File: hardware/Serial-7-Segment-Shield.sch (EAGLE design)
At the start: 32 parts, among them J1 AVR_SPI_PRG_6PTH, U1 ARDUINO_SHIELDLABEL

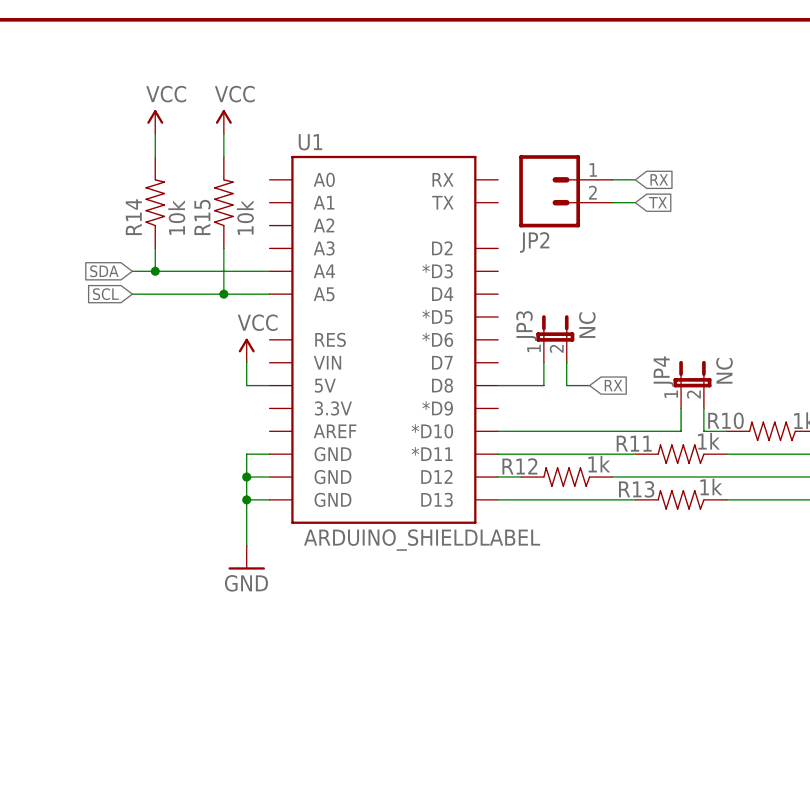
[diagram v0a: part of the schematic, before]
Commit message: commit to QC branch
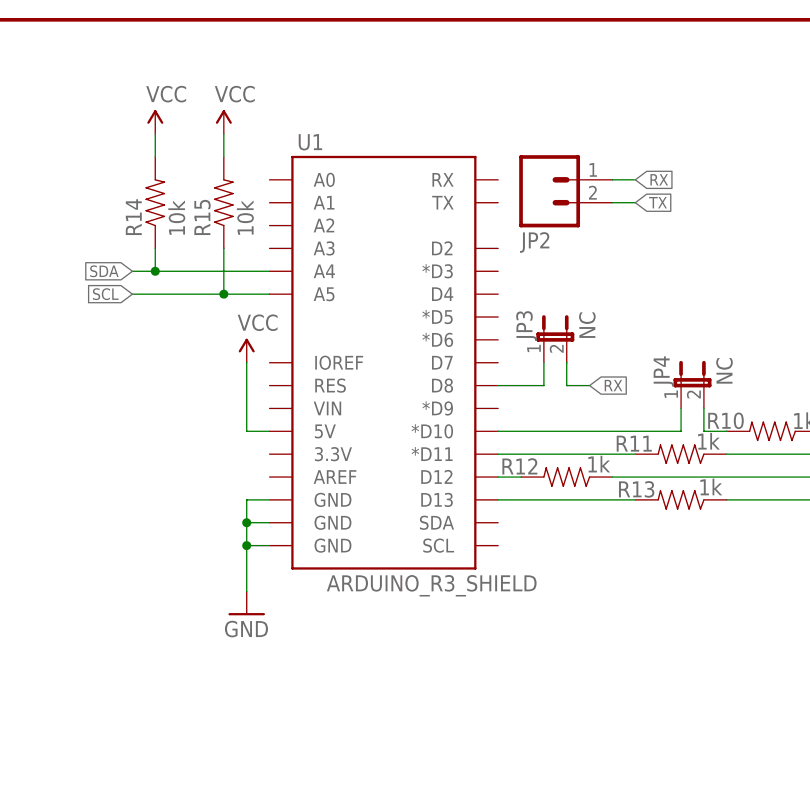
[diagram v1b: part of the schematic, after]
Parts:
- U1: value ARDUINO_SHIELDLABEL -> ARDUINO_R3_SHIELD; device SparkFun-Boards:ARDUINO_SHIELDLABEL -> SparkFun-Boards:ARDUINO_R3_SHIELD
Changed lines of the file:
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@@
 <?xml version="1.0" encoding="utf-8"?>
 <!DOCTYPE eagle SYSTEM "eagle.dtd">
-<eagle version="6.5.0">
+<eagle version="6.4">
 <drawing>
 <settings>
@@
 <part name="JP9" library="SparkFun" deviceset="FIDUCIAL" device="UFIDUCIAL"/>
 <part name="JP10" library="SparkFun" deviceset="FIDUCIAL" device="UFIDUCIAL"/>
-<part name="U1" library="SparkFun-Boards" deviceset="ARDUINO_SHIELD" device="LABEL"/>
+<part name="U1" library="SparkFun-Boards" deviceset="ARDUINO_R3_SHIELD" device=""/>
 <part name="GND5" library="SparkFun" deviceset="GND" device=""/>
 <part name="P+6" library="SparkFun" deviceset="VCC" device=""/>
@@
 <instance part="JP10" gate="G$1" x="210.82" y="33.02"/>
 <instance part="U1" gate="G$1" x="50.8" y="149.86"/>
-<instance part="GND5" gate="1" x="35.56" y="124.46"/>
+<instance part="GND5" gate="1" x="35.56" y="119.38"/>
 <instance part="P+6" gate="1" x="35.56" y="147.32"/>
 <instance part="LOGO1" gate="G$1" x="241.3" y="17.78"/>
@@
 <segment>
 <pinref part="U1" gate="G$1" pin="5V"/>
-<wire x1="38.1" y1="144.78" x2="35.56" y2="144.78" width="0.1524" layer="91"/>
+<wire x1="38.1" y1="139.7" x2="35.56" y2="139.7" width="0.1524" layer="91"/>
 <pinref part="P+6" gate="1" pin="VCC"/>
-<wire x1="35.56" y1="144.78" x2="35.56" y2="147.32" width="0.1524" layer="91"/>
+<wire x1="35.56" y1="139.7" x2="35.56" y2="147.32" width="0.1524" layer="91"/>
 </segment>
 <segment>
@@
 <segment>
 <pinref part="GND5" gate="1" pin="GND"/>
-<wire x1="35.56" y1="127" x2="35.56" y2="132.08" width="0.1524" layer="91"/>
+<wire x1="35.56" y1="121.92" x2="35.56" y2="127" width="0.1524" layer="91"/>
 <pinref part="U1" gate="G$1" pin="GND@0"/>
+<wire x1="35.56" y1="127" x2="38.1" y2="127" width="0.1524" layer="91"/>
+<wire x1="35.56" y1="127" x2="35.56" y2="129.54" width="0.1524" layer="91"/>
+<junction x="35.56" y="127"/>
+<pinref part="U1" gate="G$1" pin="GND@1"/>
+<wire x1="35.56" y1="129.54" x2="38.1" y2="129.54" width="0.1524" layer="91"/>
+<wire x1="35.56" y1="129.54" x2="35.56" y2="132.08" width="0.1524" layer="91"/>
+<junction x="35.56" y="129.54"/>
+<pinref part="U1" gate="G$1" pin="GND@2"/>
 <wire x1="35.56" y1="132.08" x2="38.1" y2="132.08" width="0.1524" layer="91"/>
-<wire x1="35.56" y1="132.08" x2="35.56" y2="134.62" width="0.1524" layer="91"/>
-<junction x="35.56" y="132.08"/>
-<pinref part="U1" gate="G$1" pin="GND@1"/>
-<wire x1="35.56" y1="134.62" x2="38.1" y2="134.62" width="0.1524" layer="91"/>
-<wire x1="35.56" y1="134.62" x2="35.56" y2="137.16" width="0.1524" layer="91"/>
-<junction x="35.56" y="134.62"/>
-<pinref part="U1" gate="G$1" pin="GND@2"/>
-<wire x1="35.56" y1="137.16" x2="38.1" y2="137.16" width="0.1524" layer="91"/>
-</segment>
-<segment>
+</segment>
+<segment>
